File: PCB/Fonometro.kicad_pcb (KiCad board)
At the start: 2 copper layers, 120 x 120 mm, 58 parts, among them J1 Conn_01x15_Male, J2 Conn_01x15_Male, J3 Power, U1 LM324, U2 LM358, U3 ESP32-DEVKIT-V1

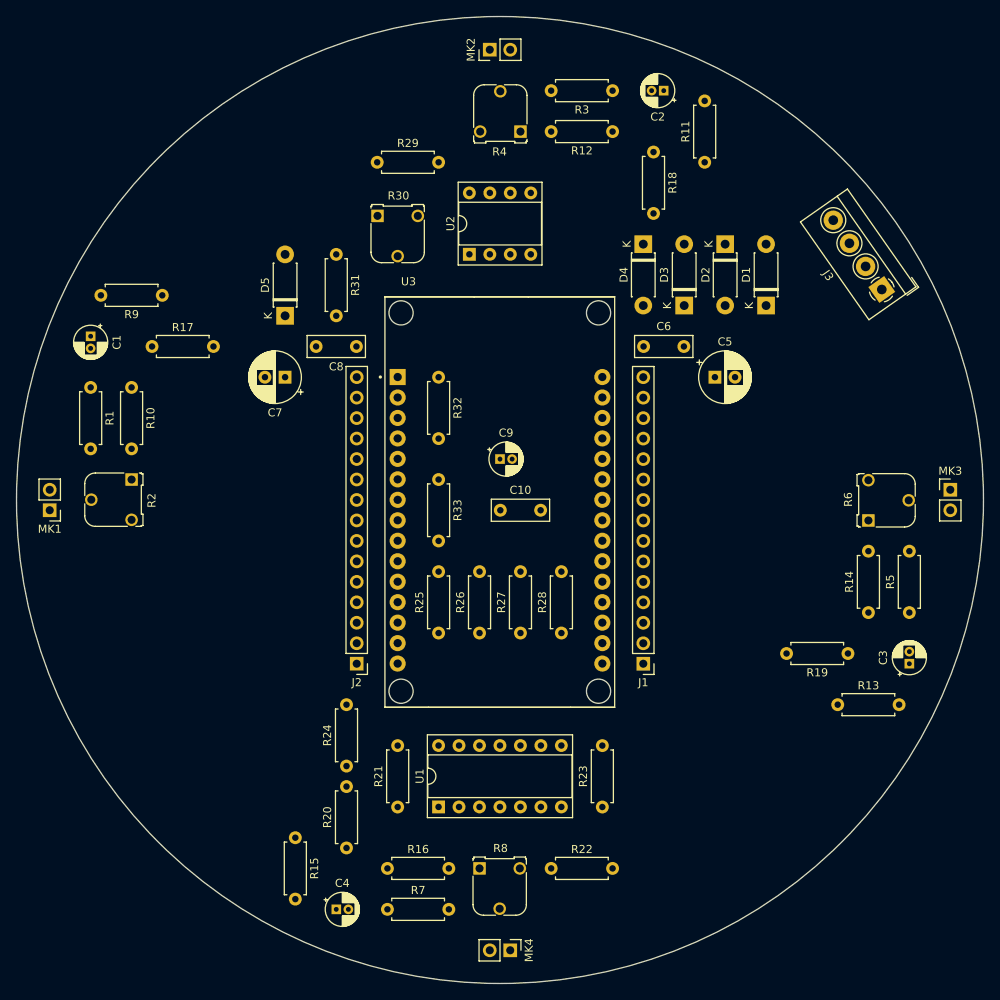
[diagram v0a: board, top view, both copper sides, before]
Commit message: feat: improved PCB layout.
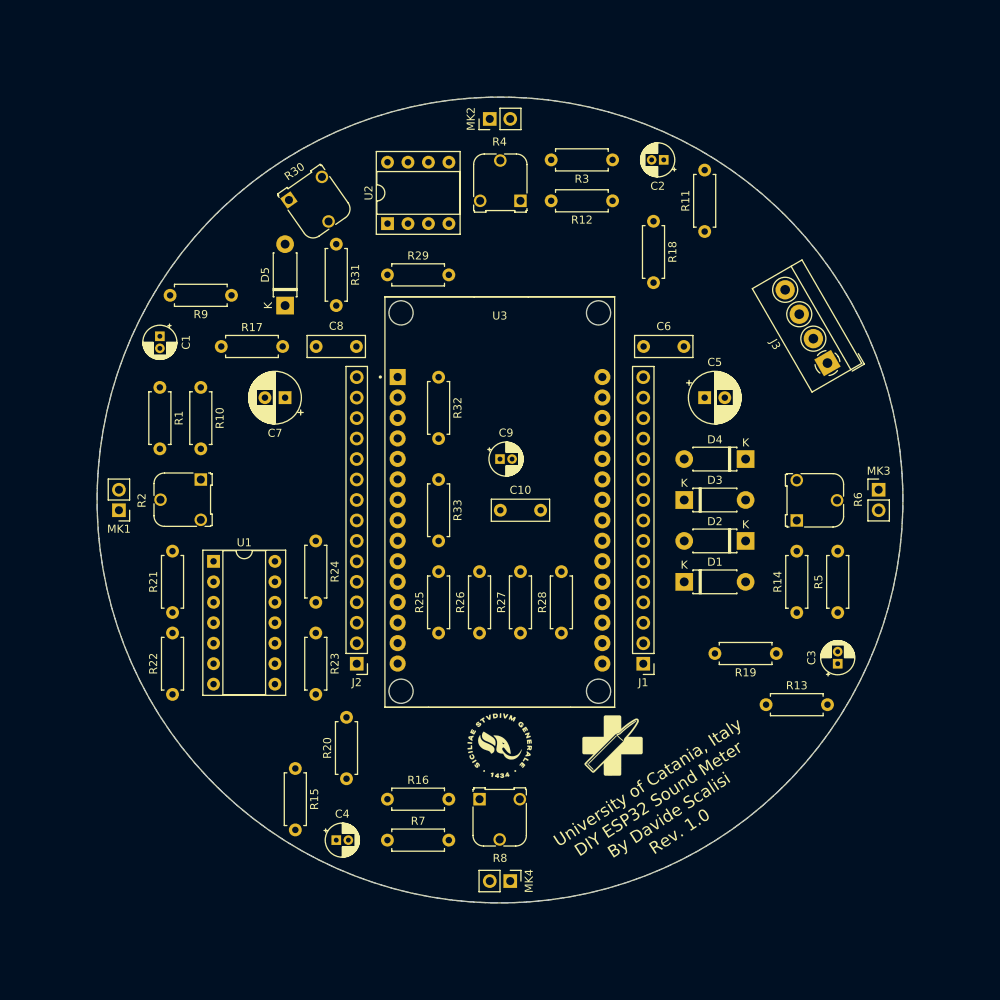
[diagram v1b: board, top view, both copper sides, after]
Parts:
- added G***: LOGO, Logos:Jugg, F.Cu at (161.3, 127.0)
- added G***: LOGO, Logos:UniCT, F.Cu at (147.3, 127.0)
- moved R22 51.7 mm to (106.7, 120.6), turned to 90 degrees
- moved R23 41.6 mm to (124.5, 113.0), turned to -90 degrees
- moved U1 41.3 mm to (111.8, 104.1), turned to 0 degrees
- moved R21 36.9 mm to (106.7, 110.5)
- moved D2 36.9 mm to (177.8, 101.6), turned to 180 degrees
- moved D1 35.8 mm to (170.2, 106.7), turned to 0 degrees
- moved D4 29.5 mm to (177.8, 91.4), turned to 180 degrees
- moved R24 28.2 mm to (124.5, 101.6), turned to -90 degrees
- moved D3 24.1 mm to (170.2, 96.5), turned to 0 degrees
- moved R29 14.0 mm to (133.3, 68.6)
- moved J3 11.3 mm to (188.0, 79.5), turned to 120 degrees
- moved R30 11.2 mm to (121.1, 59.3), turned to 35 degrees
- moved U2 10.9 mm to (133.4, 62.2)
- moved C3 8.89 mm to (189.2, 116.8)
- moved R5 8.89 mm to (189.2, 110.5)
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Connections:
- R22 pad 1: Net-(R18-Pad2) -> MIC 2
- R22 pad 2: MIC 2 -> Net-(R18-Pad2)
- R24 pad 1: Net-(R20-Pad2) -> MIC 4
- R24 pad 2: MIC 4 -> Net-(R20-Pad2)
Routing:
- added copper zone on B.Cu, net GND
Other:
- board size 120 x 120 mm -> 100 x 100 mm
- board text added: "JLCJLCJLCJLC"
- board text added: "University of Catania, Italy DIY ESP32 Sound Meter By Davide Scalisi Rev. 1.0"
